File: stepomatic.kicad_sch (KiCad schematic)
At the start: 31 parts, among them J1 I2C, J4 USB_B_Micro, Q1 MMBT3904, Q2 MMBT3904, SW1 Mode, SW2 RST, U1 HDC1080DMBR, U2 AMS1117-3.3, U3 ULN2003A, U4 CH340C, U5 28BYJ-48, U7 ESP-07

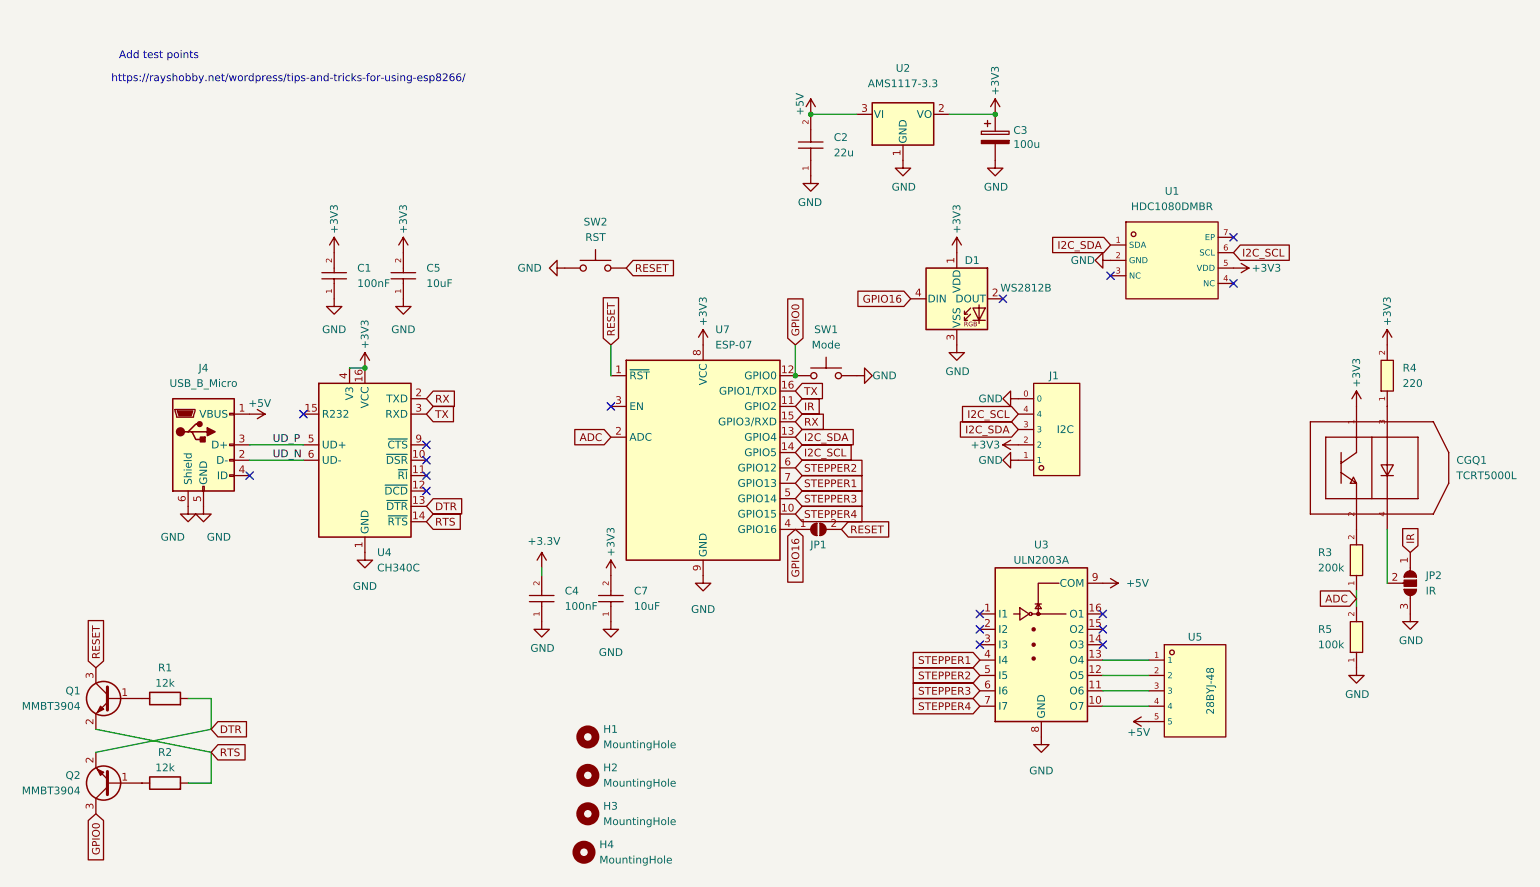
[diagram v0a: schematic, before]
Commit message: Tidy up for review
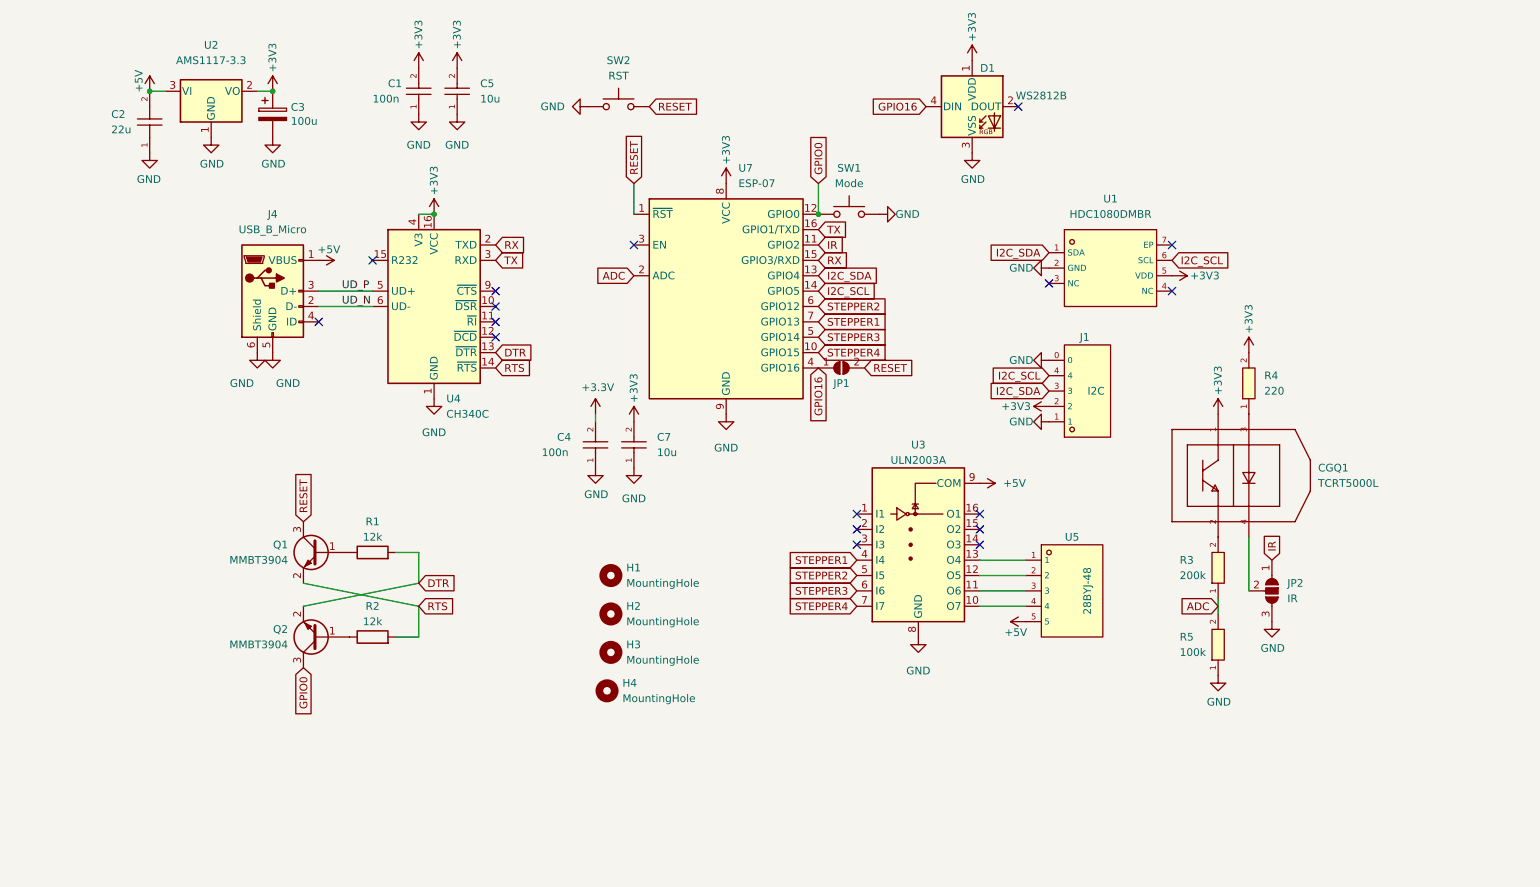
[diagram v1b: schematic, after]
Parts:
- C1, C4: value 100nF -> 100n
- C5, C7: value 10uF -> 10u
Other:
- note removed: "Add test points"
- note removed: "https://rayshobby.net/wordpress/tips-and-tricks-for-using-esp8266/"
- moved on the sheet: C1, C2, C3, C4, C5, C7, CGQ1, D1, H1, H2, H3, H4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
